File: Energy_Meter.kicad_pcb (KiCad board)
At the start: 2 copper layers, 82 x 120 mm, 121 parts, among them J1 Conn_Jack_Stereo_3.5mm_SMD_RA, J10 Conn_01x01, J2 Conn_01x04_Pin, J3 USB_C_Receptacle, J4 Conn_01x01, J5 Conn_01x01, J6 Conn_01x01, J9 3.5mm, SW3 SW_SPDT, SW4 EC11E15244G1, SW6 SW_Push, SW7 SW_Push, SW8 SW_Push, T1 ZMPT101B, U1 STM32F103C8Tx, U3 CH340G, U4 AMS1117-3.3, U5 IP5306, U6 INA226, Y1 Crystal_8MHz

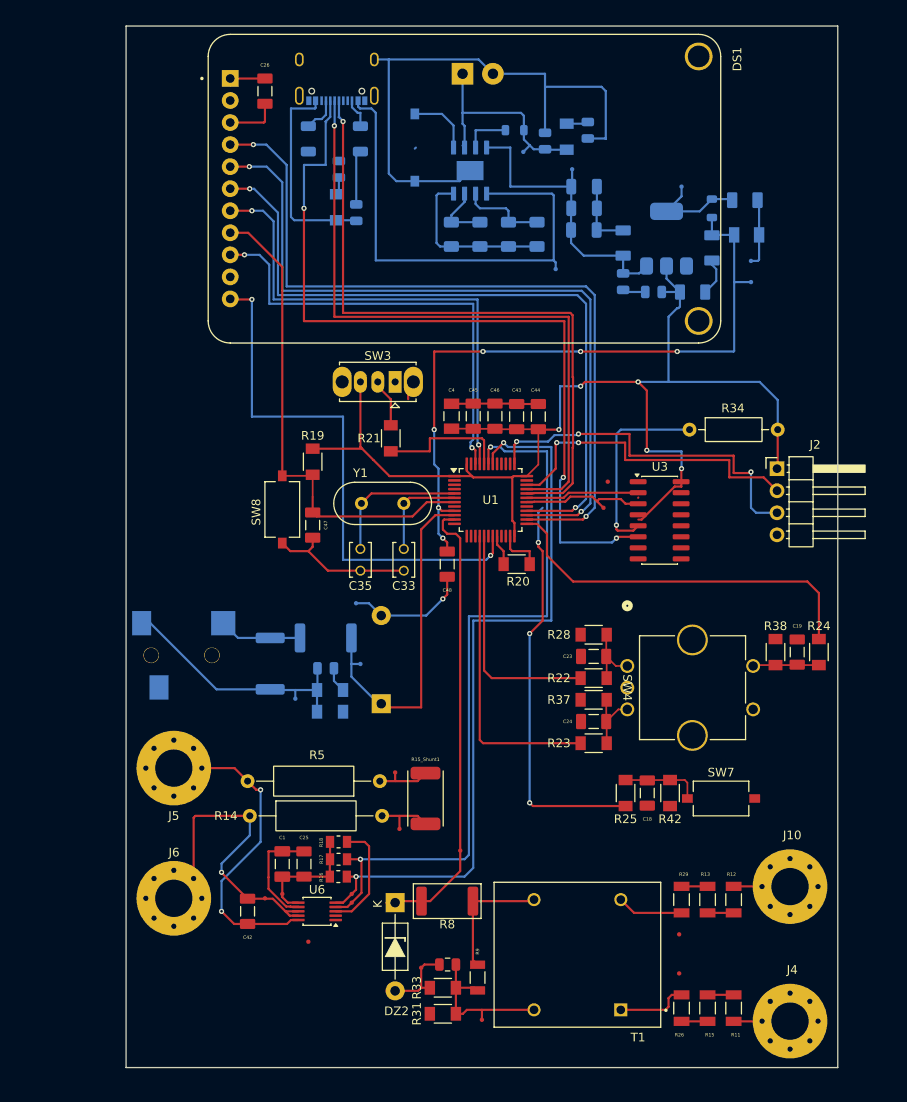
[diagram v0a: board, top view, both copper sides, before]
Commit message: update 17/07/2026
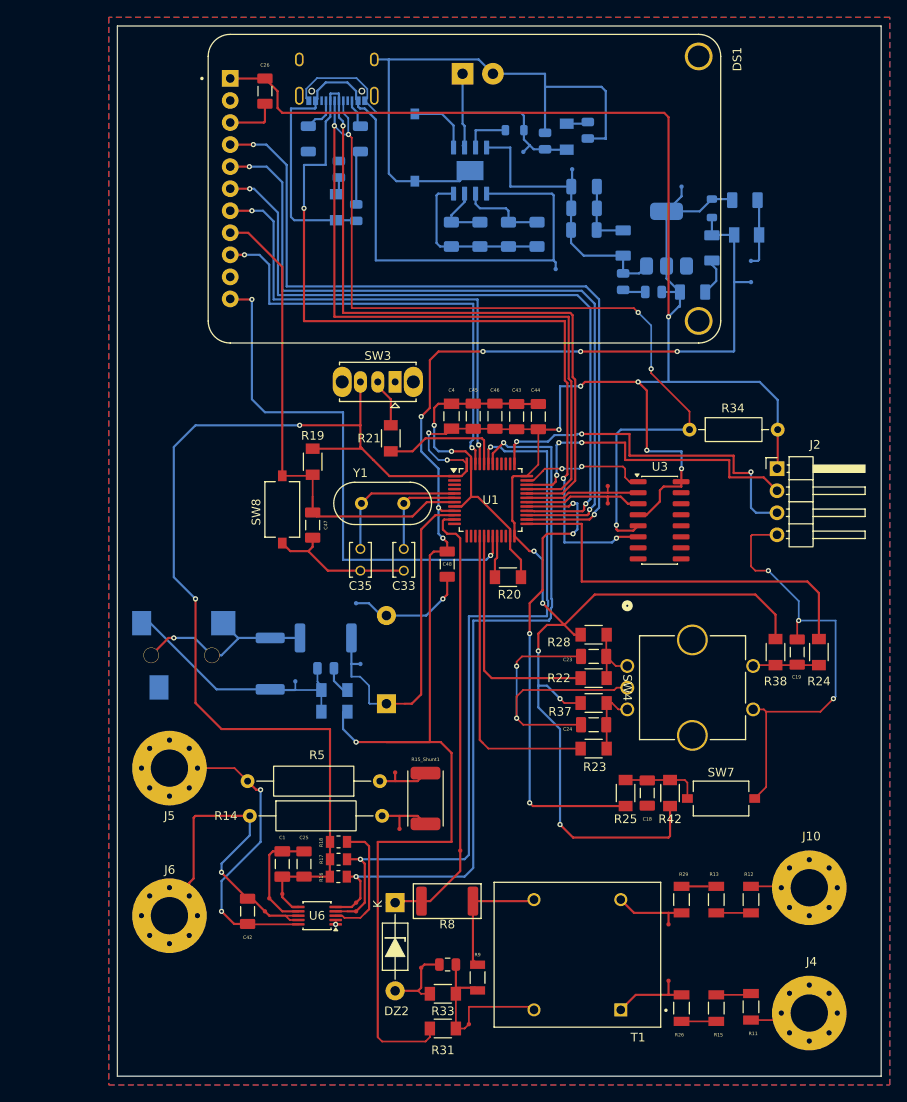
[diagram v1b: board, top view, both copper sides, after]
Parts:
- moved TP21 6.73 mm to (113.5, 120.5)
- moved J4 2.41 mm to (175.7, 133.7)
- moved J10 2.22 mm to (175.7, 119.3)
- moved J6 2.06 mm to (102.0, 122.5)
- moved R11 2.01 mm to (169.0, 133.0)
- moved R12 2.00 mm to (169.0, 120.7)
- moved TP5 2.00 mm to (116.5, 95.5), turned to 180 degrees
- moved R20 1.80 mm to (141.0, 83.5)
- moved R31 1.69 mm to (133.5, 135.5)
- moved TP16 1.68 mm to (159.5, 123.5), turned to 180 degrees
- moved TP2 1.58 mm to (136.5, 135.0)
- moved TP12 1.50 mm to (113.0, 122.0)
- moved TP13 1.49 mm to (159.5, 130.0), turned to 0 degrees
- moved TP10 1.12 mm to (123.5, 121.0)
- moved TP9 1.12 mm to (123.5, 122.0)
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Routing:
- net 3.3VD: track 169.9 -> 430.1 mm, vias 5 -> 15
- net GND: track 174.2 -> 317.9 mm, vias 1 -> 11
- net 3.3VA: track 80.2 -> 174.6 mm, vias 6 -> 7
- net /USB_C+: track 98.5 -> 174.4 mm, vias 2 -> 5
- net Net-(J1-Pad2): track 9.83 -> 22.4 mm, vias 0 -> 1
- net /RANGE: track 46.2 -> 55.8 mm, vias 3 -> 4
- net /VBUS: track 80.8 -> 88.1 mm
- net /PUSH: track 43.7 -> 46.2 mm
- net IN-: track 33.9 -> 36.3 mm
- net /USB_C-: track 169.7 -> 172.1 mm
- net Net-(C41-Pad1): track 18.6 -> 20.7 mm
- net Net-(U6-~{Alert}): track 12.9 -> 14.4 mm
- net /SDA1: track 86.1 -> 87.6 mm
- net /SCL1: track 85.6 -> 87.0 mm
- net Net-(R29-Pad2): track 7.63 -> 8.95 mm
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- added copper zone on B.Cu, net GND
- added copper zone on F.Cu, net GND
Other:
- board size 82 x 120 mm -> 88 x 121 mm

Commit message: update 17/07/2026
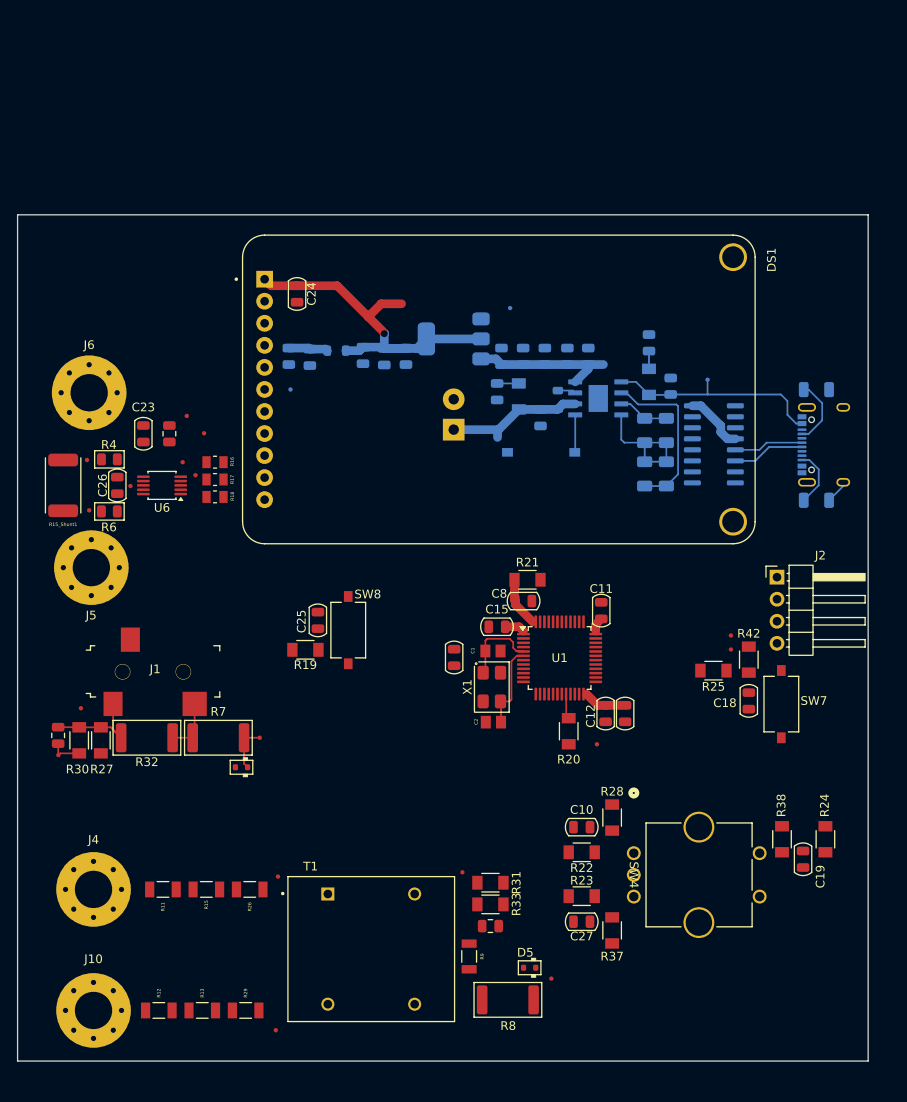
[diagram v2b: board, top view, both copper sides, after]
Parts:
- removed C33, C35: 22pF, Components_Footprint:CAPRB250W50L400T250H550
- removed C40: 10uF, PCM_SparkFun-Capacitor:C_0805_2012Metric
- removed C42, C45, C46, C47, C48: 100nF_1206_10%, Components_Footprint:CAPC3216X100N
- removed C44: 100nF_1206, Components_Footprint:CAPC3216X100N
- removed C7: 22uF, PCM_SparkFun-Capacitor:C_1206_3216Metric
- removed D7, D8: Blue, PCM_SparkFun-LED:LED_1206_3216Metric_Blue
- removed DZ1, DZ2: 1N4728A, PCM_Diode_THT_AKL:D_DO-41_SOD81_P10.16mm_Horizontal_Zener
- removed R14, R5: 10R_0.5W, Resistor_THT:R_Axial_DIN0309_L9.0mm_D3.2mm_P15.24mm_Horizontal
- removed R34: 1.5k, Resistor_THT:R_Axial_DIN0207_L6.3mm_D2.5mm_P10.16mm_Horizontal
- removed SW3: SW_SPDT, Button_Switch_THT:SW_Slide_SPDT_Straight_CK_OS102011MS2Q
- removed Y1: Crystal_8MHz, Crystal:Crystal_HC49-4H_Vertical
- added C11: 100nF_0805, PCM_Capacitor_SMD_AKL:C_0805_2012Metric, F.Cu at (151.8, 87.3)
- added C12: 100nF_0805, PCM_Capacitor_SMD_AKL:C_0805_2012Metric, F.Cu at (152.2, 99.2)
- added C14: 100nF_0805, PCM_Capacitor_SMD_AKL:C_0805_2012Metric, F.Cu at (154.5, 99.2)
- added C15: 10nF_0805, PCM_Capacitor_SMD_AKL:C_0805_2012Metric, F.Cu at (139.7, 89.2)
- added C16: 100nF_0805, PCM_Capacitor_SMD_AKL:C_0805_2012Metric, F.Cu at (134.8, 92.8)
- added C20: 100nF_0805, PCM_Capacitor_SMD_AKL:C_0805_2012Metric, B.Cu at (142.8, 58.0)
- added C21: 100nF_0805, PCM_Capacitor_SMD_AKL:C_0805_2012Metric, B.Cu at (126.8, 58.1)
- added C22: 100nF_0805, PCM_Capacitor_SMD_AKL:C_0805_2012Metric, B.Cu at (115.8, 58.0)
- added C27: 100nF_0805, PCM_Capacitor_SMD_AKL:C_0805_2012Metric, F.Cu at (149.5, 123.2)
- added C8: 100nF_0805, PCM_Capacitor_SMD_AKL:C_0805_2012Metric, F.Cu at (142.8, 86.2)
- added D1: Red, PCM_SparkFun-LED:LED_1206_3216Metric_Red, B.Cu at (156.8, 66.6)
- added D2: Red, PCM_SparkFun-LED:LED_1206_3216Metric_Red, B.Cu at (159.2, 66.6)
- added D3: Red, PCM_SparkFun-LED:LED_1206_3216Metric_Red, B.Cu at (156.8, 71.6)
- added D4: Red, PCM_SparkFun-LED:LED_1206_3216Metric_Red, B.Cu at (159.2, 71.6)
- added R4: 10R_0805, PCM_Resistor_SMD_AKL:R_0805_2012Metric, F.Cu at (95.1, 69.9)
- added R6: 10R_0805, PCM_Resistor_SMD_AKL:R_0805_2012Metric, F.Cu at (95.1, 75.9)
- added X1: SMD5032-4, PCM_Crystal_AKL:Crystal_SMD_5032-4Pin_5.0x3.2mm, F.Cu at (139.1, 96.2)
- C1: value 1uF_1206 -> 22pF_0805; footprint Components_Footprint:CAPC3216X180N -> Components_Footprint:CAPC2012X88N
- C10: value 100nF_1206_10% -> 100nF_0805; footprint Components_Footprint:CAPC3216X100N -> PCM_Capacitor_SMD_AKL:C_0805_2012Metric; moved to F.Cu
- C17: value 100nF_1206_10% -> 10nF_0805; footprint Components_Footprint:CAPC3216X100N -> PCM_Capacitor_SMD_AKL:C_0805_2012Metric
- C18, C19, C23, C24, C25, C26: value 100nF_1206_10% -> 100nF_0805; footprint Components_Footprint:CAPC3216X100N -> PCM_Capacitor_SMD_AKL:C_0805_2012Metric
- C2: value 1uF_1206 -> 22pF_0805; footprint Components_Footprint:CAPC3216X180N -> Components_Footprint:CAPC2012X88N; moved to F.Cu
- C3: value 22uF -> 1.0uF; footprint PCM_SparkFun-Capacitor:C_1206_3216Metric -> PCM_SparkFun-Capacitor:C_0805_2012Metric
- C4: value 10nF_1206 -> 22uF; footprint Components_Footprint:CAPC3216X90N -> PCM_SparkFun-Capacitor:C_0805_2012Metric; moved to B.Cu
- C43: value 100nF_1206_10% -> 10uF; footprint Components_Footprint:CAPC3216X100N -> PCM_SparkFun-Capacitor:C_0805_2012Metric
- C5: value 10nF_1206 -> 22uF; footprint Components_Footprint:CAPC3216X90N -> PCM_SparkFun-Capacitor:C_0805_2012Metric
- C6: value 22uF -> 1.0uF; footprint PCM_SparkFun-Capacitor:C_1206_3216Metric -> PCM_SparkFun-Capacitor:C_0805_2012Metric; moved to F.Cu
- C9: value 100nF_1206_10% -> 22uF; footprint Components_Footprint:CAPC3216X100N -> PCM_SparkFun-Capacitor:C_0805_2012Metric
- D5, D6: value Blue -> PESD5Z3.3; footprint PCM_SparkFun-LED:LED_1206_3216Metric_Blue -> PCM_Diode_SMD_AKL:D_SOD-523; moved to F.Cu
- J1, R27, R30, R32, R7, TP14, TP4, TP5, TP6: moved to F.Cu
- U3: moved to B.Cu
- moved D5 85.0 mm to (143.5, 128.5), turned to 180 degrees
- moved J4 83.7 mm to (93.2, 119.5), turned to -90 degrees
- moved J10 83.7 mm to (93.2, 133.4), turned to -90 degrees
- moved R12 69.4 mm to (100.8, 133.4), turned to 0 degrees
- moved R11 69.1 mm to (101.2, 119.5), turned to 0 degrees
- moved C10 67.5 mm to (149.5, 112.3), turned to 180 degrees
- moved D6 67.3 mm to (110.3, 105.4), turned to 180 degrees
- moved R1 67.0 mm to (176.5, 74.6), turned to 180 degrees
- moved C2 66.8 mm to (139.3, 100.2), turned to 180 degrees
- moved J3 66.2 mm to (174.5, 68.2), turned to -90 degrees
- moved R2 65.3 mm to (176.5, 61.9), turned to 180 degrees
- moved C43 64.3 mm to (89.2, 101.7), turned to -90 degrees
- moved J6 61.0 mm to (92.8, 62.2)
- moved R13 60.6 mm to (105.8, 133.4), turned to 0 degrees
- moved R15 60.3 mm to (106.2, 119.5), turned to 0 degrees
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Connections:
- C1 pad 1: 3.3VD -> GND
- C1 pad 2: GND -> /HSE_IN
- C10 pad 1: 5V -> Net-(C10-Pad1)
- C2 pad 1: 3.3VD -> /HSE_OUT
- C23 pad 1: Net-(C23-Pad1) -> 3.3VD
- C24 pad 1: Net-(C24-Pad1) -> 3.3VD
- C25 pad 1: 3.3VD -> /TFT_RST
- C26 pad 1: 3.3VD -> IN+
- C26 pad 2: GND -> IN-
- C3 pad 1: 5V -> 3.3VD
- C4 pad 1: 3.3VD -> 5V
- C43 pad 1: 3.3VD -> Net-(C43-Pad1)
- C5 pad 1: 3.3VA -> 5V
- C6 pad 1: 5V -> 3.3VD
- C9 pad 1: 3.3VD -> 5V
- D5 pad 1: Net-(D5-K) -> ADC2
- D5 pad 2: Net-(D5-A) -> GND
- D6 pad 1: Net-(D5-A) -> ADC1
- D6 pad 2: Net-(D5-K) -> GND
- J1 pad 1: Net-(C40-Pad1) -> Net-(C43-Pad1)
- R21 pad 1: Net-(SW3-B) -> 3.3VD
- R22 pad 2: Net-(C23-Pad1) -> Net-(C10-Pad1)
- R23 pad 1: Net-(C24-Pad1) -> Net-(C27-Pad1)
- R27 pad 2: Net-(C40-Pad1) -> Net-(C43-Pad1)
- R28 pad 2: Net-(C23-Pad1) -> Net-(C10-Pad1)
- R30 pad 1: Net-(C40-Pad1) -> Net-(C43-Pad1)
- R32 pad 1: Net-(C40-Pad1) -> Net-(C43-Pad1)
- R37 pad 2: Net-(C24-Pad1) -> Net-(C27-Pad1)
- SW4 pad A: Net-(C23-Pad1) -> Net-(C10-Pad1)
- SW4 pad B: Net-(C24-Pad1) -> Net-(C27-Pad1)
- TP5 pad 1: Net-(C40-Pad1) -> Net-(C43-Pad1)
- U1 pad 32: /USB_C- -> unconnected-(U1-PA11-Pad32)
- U1 pad 33: /USB_C+ -> unconnected-(U1-PA12-Pad33)
- U5 pad 3: Net-(D5-K) -> Net-(D1-K)
- U5 pad 4: Net-(D5-A) -> Net-(D1-A)
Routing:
- net 3.3VD: track 430.1 -> 62.8 mm, vias 15 -> 1
- net GND: track 317.9 -> 6.56 mm, vias 11 -> 0
- net 3.3VA: track 174.6 -> 4.56 mm, vias 7 -> 0
- net /USB_C+: track 174.4 -> 8.02 mm, vias 5 -> 0
- net /USB_C-: track 172.1 -> 8.34 mm, vias 4 -> 0
- net /TFT_SCK: track 91.2 -> 0.00 mm, vias 2 -> 0
- net /SDA1: track 87.6 -> 0.00 mm, vias 2 -> 0
- net /TFT_MISO: track 87.6 -> 0.00 mm, vias 2 -> 0
- net /SCL1: track 87.0 -> 0.00 mm, vias 2 -> 0
- net /TFT_MOSI: track 83.0 -> 0.00 mm, vias 2 -> 0
- net /VBUS: track 88.1 -> 25.5 mm
- net /TFT_BLK: track 61.7 -> 0.00 mm, vias 2 -> 0
- net /TFT_RST: track 57.5 -> 0.00 mm
- net /TFT_CS: track 57.1 -> 0.00 mm, vias 2 -> 0
- net /RANGE: track 55.8 -> 0.00 mm, vias 4 -> 0
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- removed copper zone on B.Cu, net GND
- removed copper zone on F.Cu, net GND
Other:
- board size 88 x 121 mm -> 98 x 97.5 mm
